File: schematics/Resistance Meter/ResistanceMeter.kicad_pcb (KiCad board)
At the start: 2 copper layers, 53.3 x 54.6 mm, 29 parts, among them J1 Conn_01x01_Female, J2 Conn_01x01_Female, J3 Conn_01x16_Female, J4 Conn_01x08_Male, J5 Conn_01x06_Male, J6 Conn_01x10_Male, J7 Conn_01x08_Male, Q1 IRF540N, Q2 IRF540N, SW1 SW_Push, SW2 SW_Push

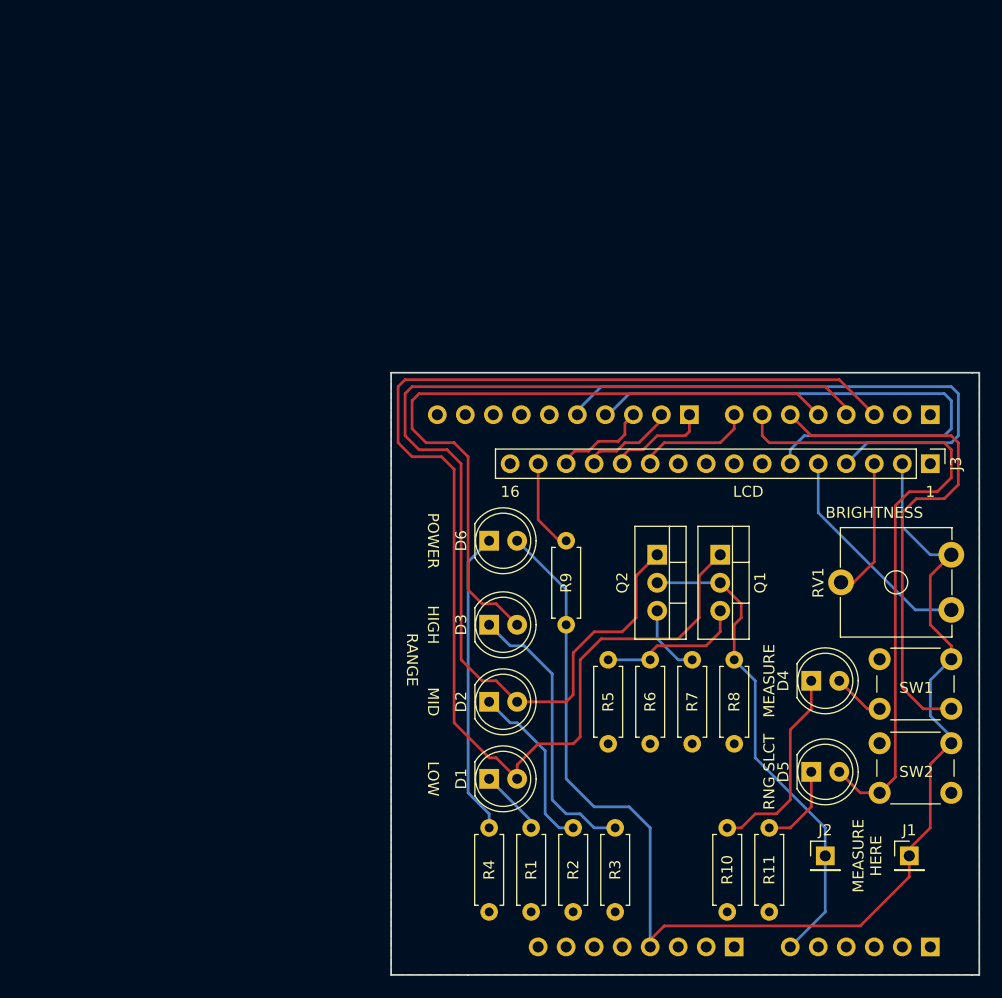
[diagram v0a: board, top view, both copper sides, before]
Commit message: Revise the project's PCB design
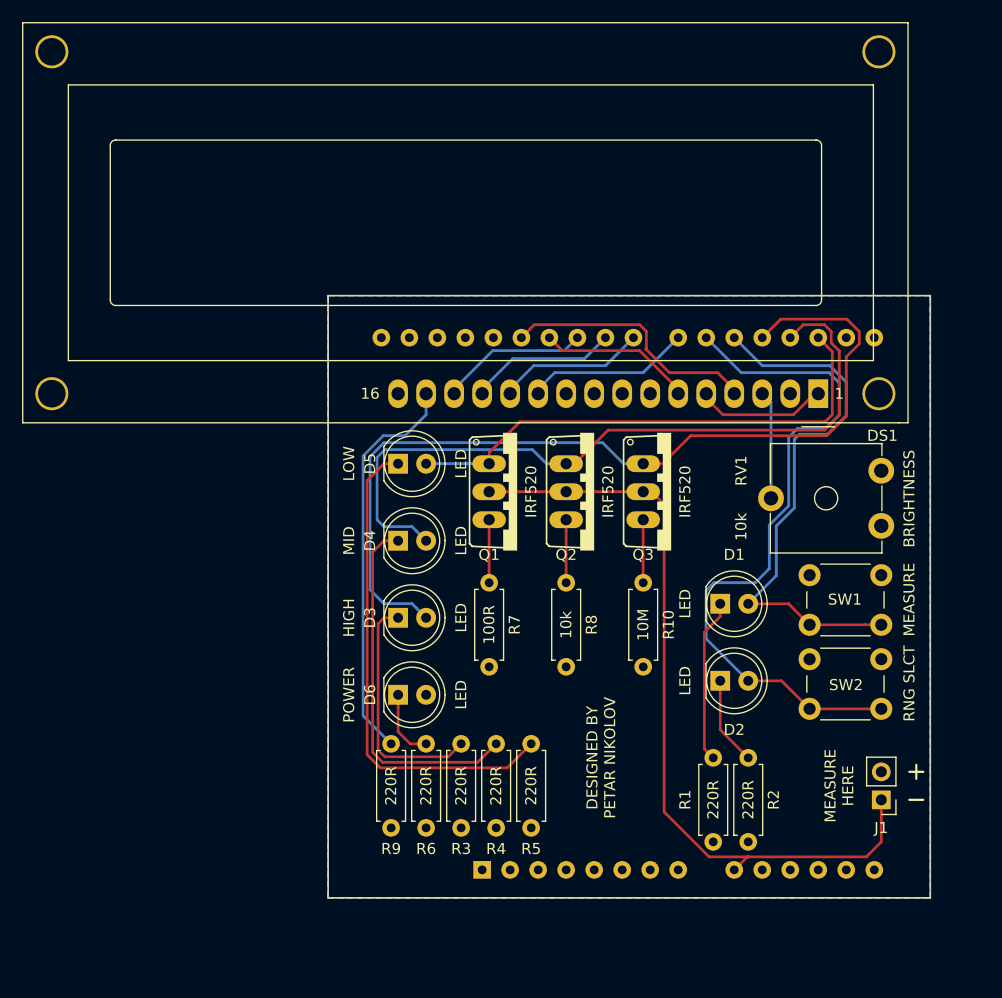
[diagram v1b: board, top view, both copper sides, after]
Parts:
- removed J2: Conn_01x01_Female, Socket_Strips:Socket_Strip_Straight_1x01_Pitch2.54mm
- removed J3: Conn_01x16_Female, Socket_Strips:Socket_Strip_Straight_1x16_Pitch2.54mm
- removed J4, J7: Conn_01x08_Male, Pin_Headers:Pin_Header_Straight_1x08_Pitch2.54mm
- removed J5: Conn_01x06_Male, Pin_Headers:Pin_Header_Straight_1x06_Pitch2.54mm
- removed J6: Conn_01x10_Male, Pin_Headers:Pin_Header_Straight_1x10_Pitch2.54mm
- removed R11: 220, Resistors_THT:R_Axial_DIN0207_L6.3mm_D2.5mm_P7.62mm_Horizontal
- added A1: Arduino_UNO_R3, Modules:Arduino_UNO_R3, B.Cu at (136.5, 109.9)
- added DS1: NDS1602A, Displays:WC1602A, F.Cu at (167.0, 66.7)
- added Q3: IRF520, IRF520:TO220BV, F.Cu at (153.7, 75.6)
- J1: value Conn_01x01_Female -> Conn_01x02_Male; footprint Socket_Strips:Socket_Strip_Straight_1x01_Pitch2.54mm -> Pin_Headers:Pin_Header_Straight_1x02_Pitch2.54mm
- Q1, Q2: value IRF540N -> IRF520; footprint TO_SOT_Packages_THT:TO-220-3_Vertical -> IRF520:TO220BV
- R1, R2, R3, R4, R5, R6, R9: value 220 -> 220R
- R10: value 220 -> 10M
- R7: value 10k -> 100R
- R8: value 10M -> 10k
- moved D5 46.7 mm to (128.9, 73.0)
- moved D4 39.6 mm to (128.9, 80.0)
- moved D1 26.3 mm to (158.1, 85.7)
- moved R9 24.3 mm to (128.3, 98.4)
- moved R10 23.5 mm to (151.1, 83.8)
- moved R6 21.7 mm to (131.4, 98.4)
- moved D2 21.0 mm to (158.1, 92.7)
- moved R7 19.7 mm to (137.2, 83.8)
- moved Q1 19.3 mm to (139.7, 75.6)
- moved R1 17.7 mm to (157.5, 99.7)
- moved R2 17.1 mm to (160.7, 99.7)
- moved R8 16.8 mm to (144.1, 83.8)
- moved D6 16.2 mm to (128.9, 94.0)
- moved R3 15.9 mm to (134.6, 98.4)
- moved R5 10.3 mm to (141.0, 98.4)
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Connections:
- net Earth renamed GND
- D1 pad 2: /b2 -> Net-(A1-Pad20)
- D2 pad 2: /b3 -> Net-(A1-Pad21)
- D3 pad 2: /b4 -> Net-(A1-Pad19)
- D4 pad 2: /b5 -> Net-(A1-Pad18)
- D5 pad 2: /b6 -> Net-(A1-Pad17)
- J1 pad 1: +5V -> /ANALOG_INPUT
- R10 pad 1: Net-(D4-Pad1) -> Net-(Q3-PadS)
- R4 pad 1: Net-(D6-Pad1) -> Net-(D4-Pad1)
- R5 pad 1: Net-(Q1-Pad3) -> Net-(D5-Pad1)
- R6 pad 1: Net-(Q1-Pad3) -> Net-(D6-Pad1)
- R7 pad 1: Net-(Q2-Pad3) -> Net-(Q1-PadS)
- R8 pad 1: /ANALOG_INPUT -> Net-(Q2-PadS)
- R9 pad 1: /a15 -> Net-(DS1-Pad15)
- RV1 pad 2: /a3 -> Net-(DS1-Pad3)
- SW1 pad 1: /b5 -> Net-(A1-Pad20)
- SW2 pad 1: /b6 -> Net-(A1-Pad21)
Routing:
- net /b2: track 120.6 -> 0.00 mm
- net +5V: track 115.3 -> 0.00 mm
- net /b3: track 98.8 -> 0.00 mm
- net Net-(A1-Pad19): track 0.00 -> 82.6 mm
- net Net-(A1-Pad18): track 0.00 -> 67.8 mm
- net /b4: track 64.4 -> 0.00 mm
- net Net-(A1-Pad21): track 0.00 -> 64.2 mm
- net /b6: track 59.3 -> 0.00 mm
- net /b5: track 52.8 -> 0.00 mm
- net /a6: track 51.6 -> 0.00 mm
- net /a4: track 51.1 -> 0.00 mm
- net Net-(A1-Pad20): track 0.00 -> 49.9 mm
- net Net-(A1-Pad17): track 0.00 -> 46.8 mm
- net Net-(D5-Pad1): track 7.77 -> 44.6 mm
- net Net-(DS1-Pad15): track 0.00 -> 36.3 mm
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- added copper zone on F.Cu, net +5V
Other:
- board size 53.3 x 54.6 mm -> 54.6 x 54.6 mm
- board text added: "Arduino Uno R3"
- board text removed: "LCD"
- board text removed: "RANGE"
